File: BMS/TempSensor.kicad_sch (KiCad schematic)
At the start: 15 parts, among them U10 TMP1075D, U11 TMP1075D, U6 TMP1075D, U7 TMP1075D, U8 TMP1075D, U9 TMP1075D

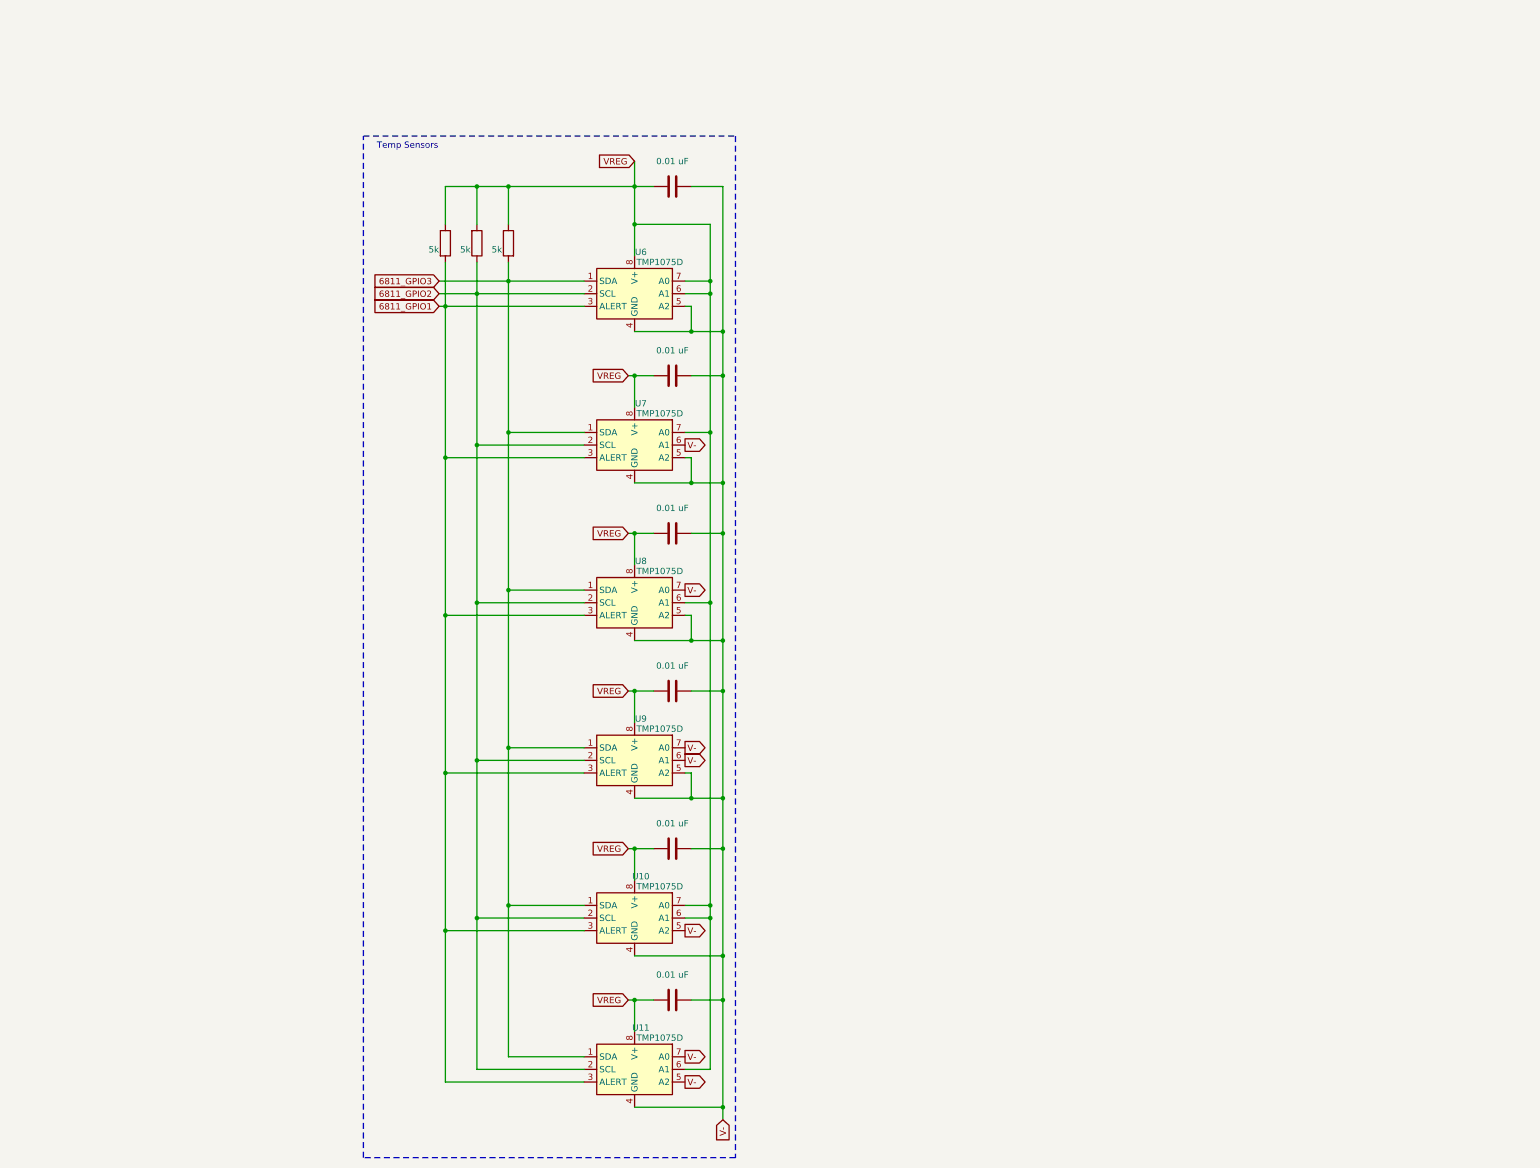
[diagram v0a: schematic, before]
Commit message: full prototype schematic
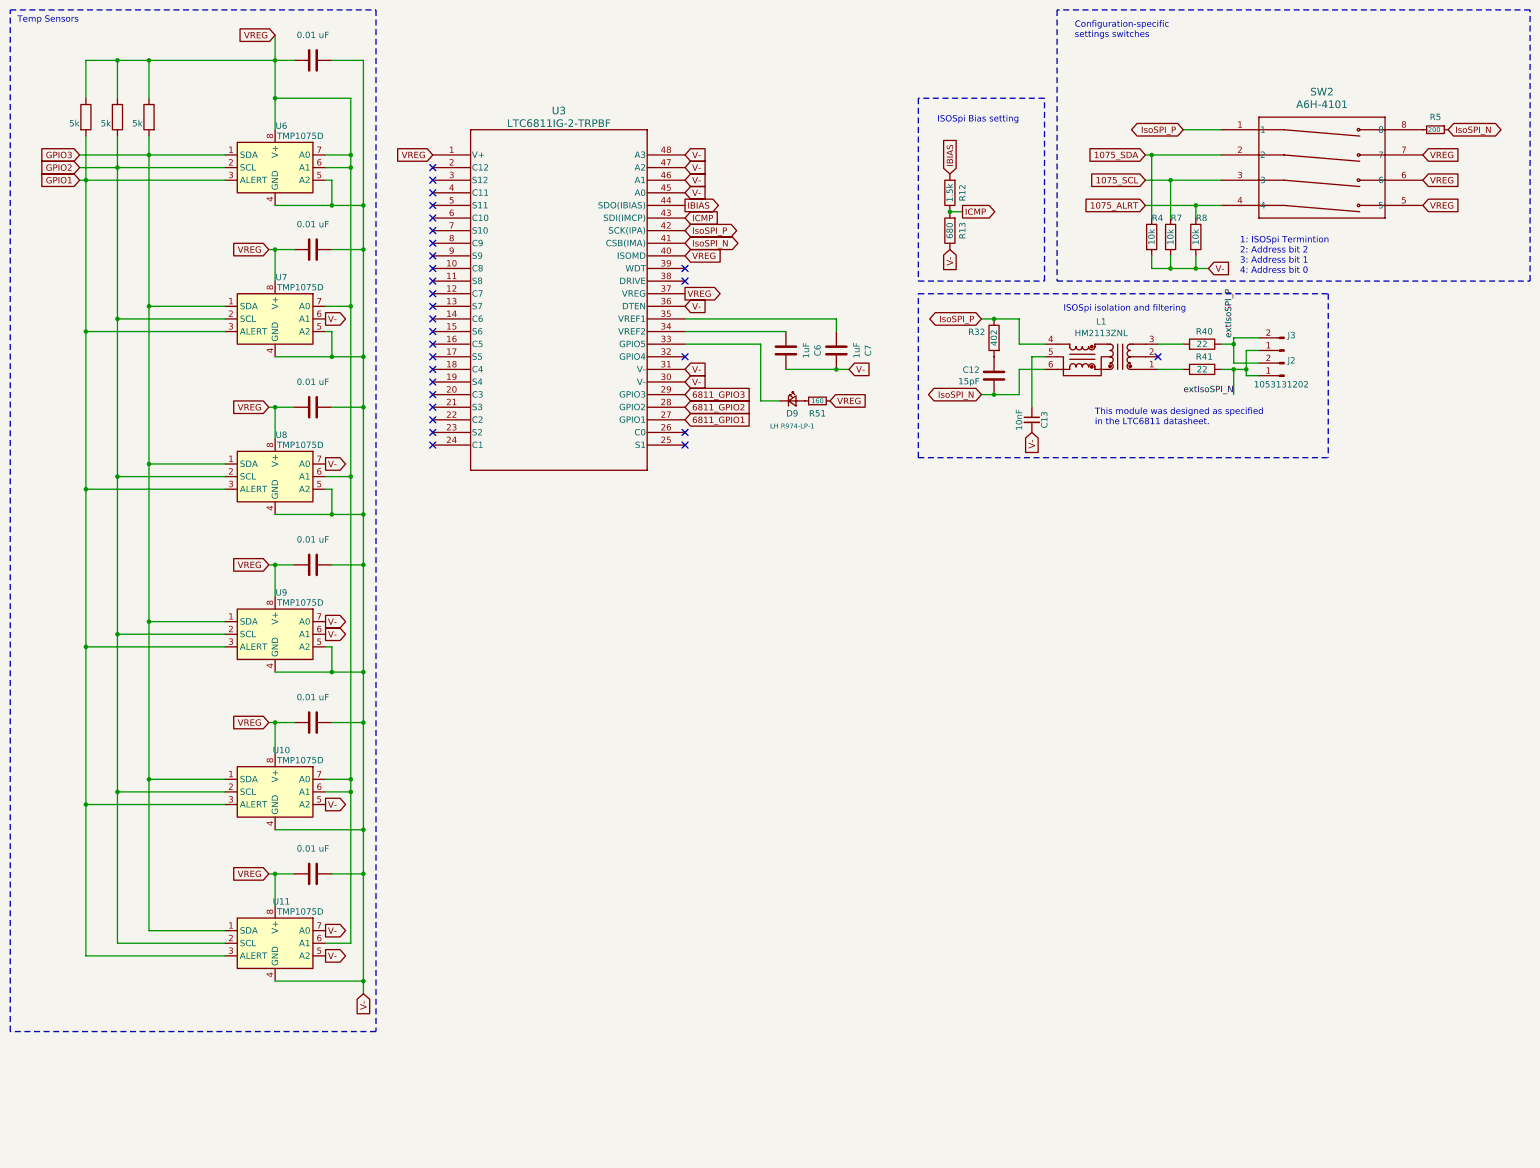
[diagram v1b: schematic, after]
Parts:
- added C12: 15pF, Capacitor_SMD:C_0805_2012Metric_Pad1.18x1.45mm_HandSolder, symbol Device:C
- added C13: 10nF, Capacitor_SMD:C_0805_2012Metric_Pad1.18x1.45mm_HandSolder, symbol Device:C_Small
- added C6, C7: 1uF, Capacitor_SMD:C_0805_2012Metric_Pad1.18x1.45mm_HandSolder, symbol Device:C
- added D9: LH R974-LP-1, LED_SMD:LED_0805_2012Metric_Pad1.15x1.40mm_HandSolder, symbol Device:LED_Small
- added J2, J3: 1053131202, Connector_Molex:Molex_Nano-Fit_105313-xx02_1x02_P2.50mm_Horizontal, symbol Connector:Conn_01x02_Pin
- added L1: HM2113ZNL, FS_3_Global_Footprint_Library:HM2113ZNLT, symbol FSSymbols:HM2113ZNL
- added R12: 1.5k, Resistor_SMD:R_0805_2012Metric_Pad1.20x1.40mm_HandSolder, symbol Device:R
- added R13: 680, Resistor_SMD:R_0805_2012Metric_Pad1.20x1.40mm_HandSolder, symbol Device:R
- added R32: 402, Resistor_SMD:R_0805_2012Metric_Pad1.20x1.40mm_HandSolder, symbol Device:R
- added R4, R7, R8: 10k, Resistor_SMD:R_0805_2012Metric_Pad1.20x1.40mm_HandSolder, symbol Device:R
- added R40, R41: 22, Resistor_SMD:R_0805_2012Metric_Pad1.20x1.40mm_HandSolder, symbol Device:R
- added R5: 200, Resistor_SMD:R_0805_2012Metric_Pad1.20x1.40mm_HandSolder, symbol Device:R_Small
- added R51: 160, Resistor_SMD:R_0805_2012Metric_Pad1.20x1.40mm_HandSolder, symbol Device:R_Small
- added SW2: A6H-4101, FS_3_Global_Footprint_Library:SW_A6H-4101_OMR, symbol FS_3_Global_Symbol_Library:A6H-4101
- added U3: LTC6811IG-2-TRPBF, FS_3_Global_Footprint_Library:LTC6811-2, symbol FS_3_Global_Symbol_Library:LTC6811IG-2-TRPBF
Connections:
- net 6811_GPIO1: now also U3.27 (GPIO1); no longer PU_ALRT.2, U10.3 (ALERT), U11.3 (ALERT), U6.3 (ALERT), U7.3 (ALERT), U8.3 (ALERT), U9.3 (ALERT)
- net 6811_GPIO2: now also U3.28 (GPIO2); no longer RPU_SCL.1, U10.2 (SCL), U11.2 (SCL), U6.2 (SCL), U7.2 (SCL), U8.2 (SCL), U9.2 (SCL)
- net 6811_GPIO3: now also U3.29 (GPIO3); no longer PU_SDA.2, U10.1 (SDA), U11.1 (SDA), U6.1 (SDA), U7.1 (SDA), U8.1 (SDA), U9.1 (SDA)
- net V-: now also C13.2, C6.1, C7.1, R13.1, R4.2, R7.2, R8.2, U3.30 (V-), U3.31 (V-), U3.36 (DTEN), U3.45 (A0), U3.46 (A1), U3.47 (A2), U3.48 (A3)
- net VREG: now also R51.2, SW2.5, SW2.6, SW2.7, U3.1 (V+), U3.37 (VREG), U3.40 (ISOMD)
- new net: C7.2, U3.35 (VREF1)
- new net: C6.2, U3.34 (VREF2)
- new net: L1.1, R41.2
- new net: L1.3, R40.2
- new net: C13.1, L1.5
- new net: C12.2, R32.2
- new net: D9.1 (K), U3.33 (GPIO5)
- new net: D9.2 (A), R51.1
- new net: R5.2, SW2.8
- new net 1075_ALRT: R8.1, SW2.4
- new net 1075_SCL: R7.1, SW2.3
- new net 1075_SDA: R4.1, SW2.2
- new net GPIO1: PU_ALRT.2, U10.3 (ALERT), U11.3 (ALERT), U6.3 (ALERT), U7.3 (ALERT), U8.3 (ALERT), U9.3 (ALERT)
- new net GPIO2: RPU_SCL.1, U10.2 (SCL), U11.2 (SCL), U6.2 (SCL), U7.2 (SCL), U8.2 (SCL), U9.2 (SCL)
- new net GPIO3: PU_SDA.2, U10.1 (SDA), U11.1 (SDA), U6.1 (SDA), U7.1 (SDA), U8.1 (SDA), U9.1 (SDA)
- new net IBIAS: R12.2, U3.44 (SDO(IBIAS))
- new net ICMP: R12.1, R13.2, U3.43 (SDI(IMCP))
- new net IsoSPI_N: C12.1, L1.6, R5.1, U3.41 (CSB(IMA))
- new net IsoSPI_P: L1.4, R32.1, SW2.1, U3.42 (SCK(IPA))
- new net extIsoSPI_N: J2.1 (Pin_1), J3.1 (Pin_1), R41.1
- new net extIsoSPI_P: J2.2 (Pin_2), J3.2 (Pin_2), R40.1
- no-connect marks 0 -> 29
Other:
- note added: "1: ISOSpi Termintion 2: Address bit 2 3: Address bit 1 4: Address bit 0"
- note added: "Configuration-specific settings switches"
- note added: "ISOSpi Bias setting"
- note added: "ISOSpi isolation and filtering"
- note added: "This module was designed as specified in the LTC6811 datasheet."
- moved on the sheet: U10, U11, U6, U7, U8, U9
